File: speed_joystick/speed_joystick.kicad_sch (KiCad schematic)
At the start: 10 parts, among them J1 Conn_01x07, J2 Conn_01x04, SW1 JS5208, U1 Teensy3.2

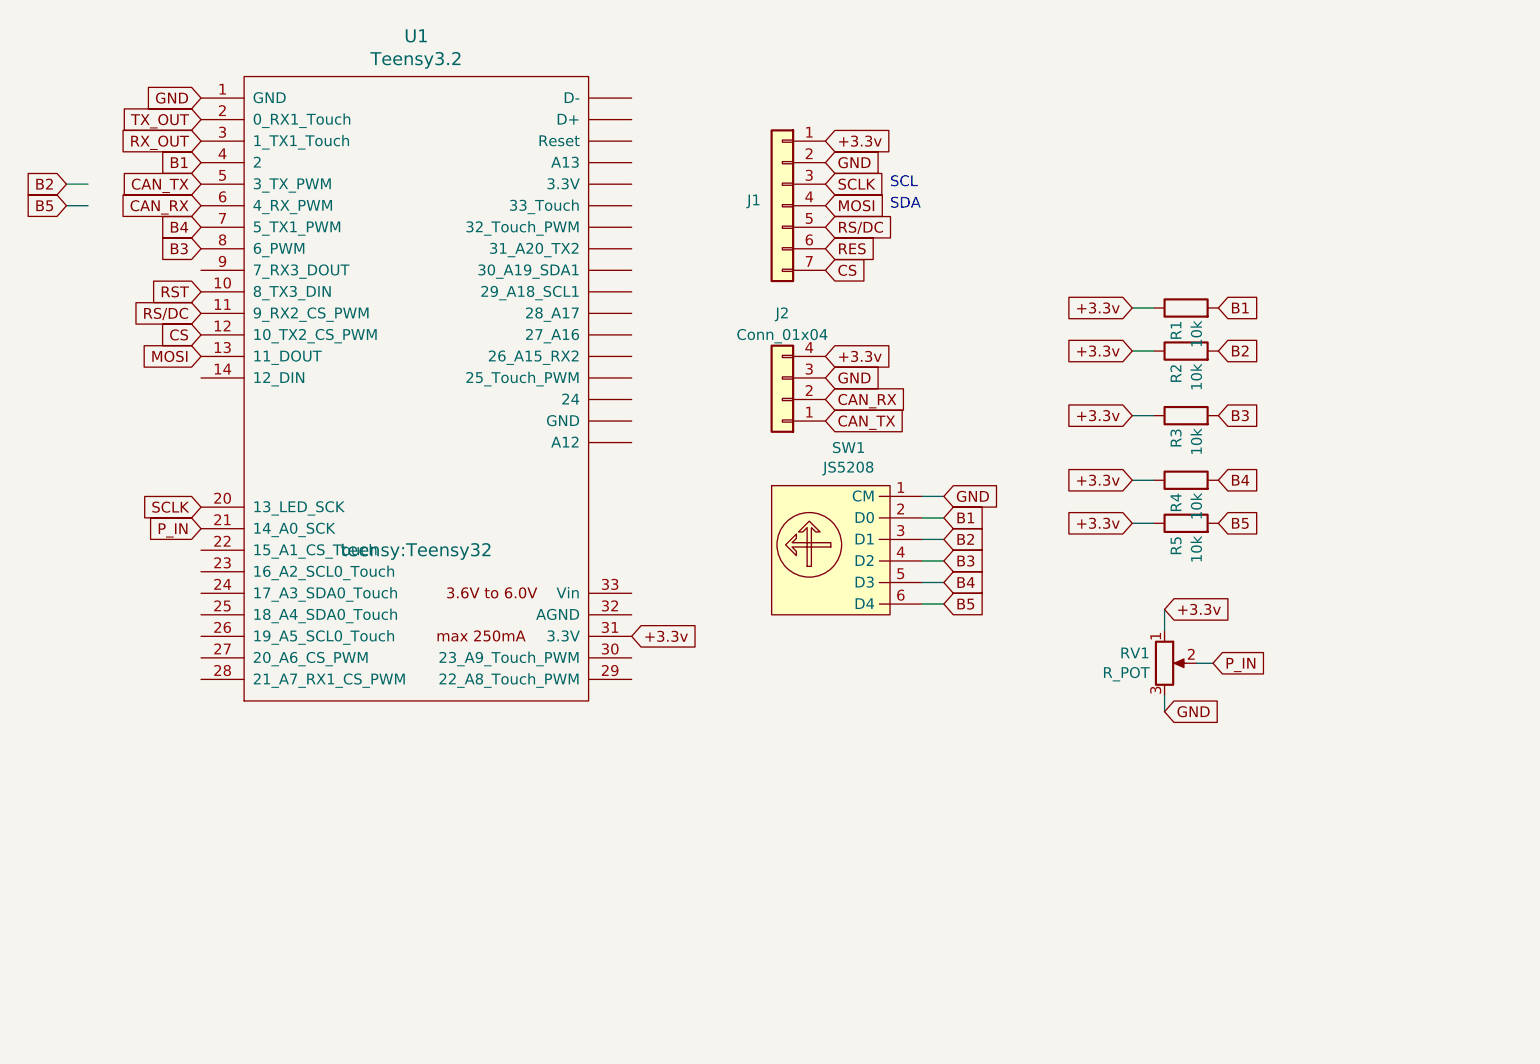
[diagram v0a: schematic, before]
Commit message: pcb work
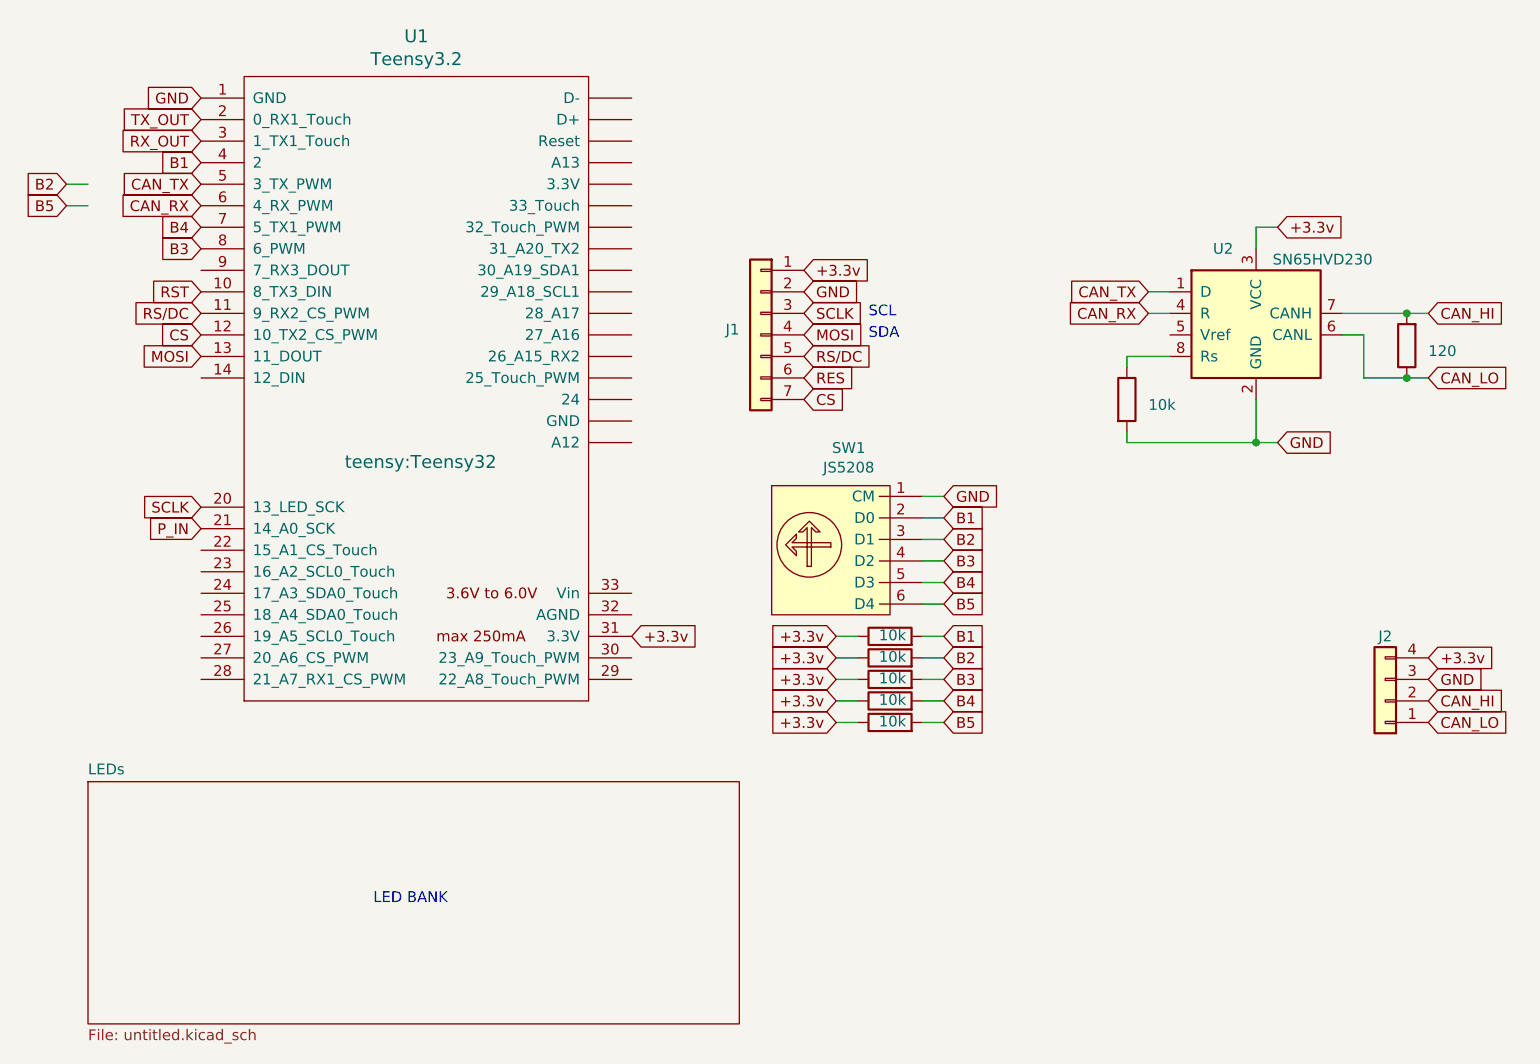
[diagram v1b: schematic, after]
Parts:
- removed RV1: R_POT, Potentiometer_SMD:slide_pot, symbol speed_joystick-rescue:R_POT-Device
- added R6, R7: 10k, Resistor_SMD:R_0805_2012Metric, symbol Device:R
- added U2: SN65HVD230, Package_SO:SOIC-8_3.9x4.9mm_P1.27mm, symbol Interface_CAN_LIN:SN65HVD230
- J2: footprint (none) -> Connector_PinSocket_2.54mm:my_4_tab_edge
- R3: value 10k -> 120; Group# 11 -> (none); P/N 755-ESR10EZPF5102 -> (none)
- SW1: footprint Button_Switch_Keyboard:Joy_switch -> JS5208:SW_JS5208
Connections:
- net +3.3v: now also R6.1, U2.3 (VCC); no longer R3.1
- net B1: now also R6.2; no longer R1.2
- net B2: now also R5.2; no longer R2.2
- net B3: now also R4.2; no longer R3.2
- net B4: now also R2.2; no longer R4.2
- net B5: now also R1.2; no longer R5.2
- net CAN_RX: now also U2.4 (R); no longer J2.2 (Pin_2)
- net CAN_TX: now also U2.1 (D); no longer J2.1 (Pin_1)
- net GND: now also R7.2, U2.2 (GND)
- new net: R7.1, U2.8 (Rs)
- new net CAN_HI: J2.2 (Pin_2), R3.2, U2.7 (CANH)
- new net CAN_LO: J2.1 (Pin_1), R3.1, U2.6 (CANL)
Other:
- added sheet LEDs (untitled.kicad_sch)
- note added: "LED BANK"
- moved on the sheet: J1, J2

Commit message: work on speed_joystick pcb
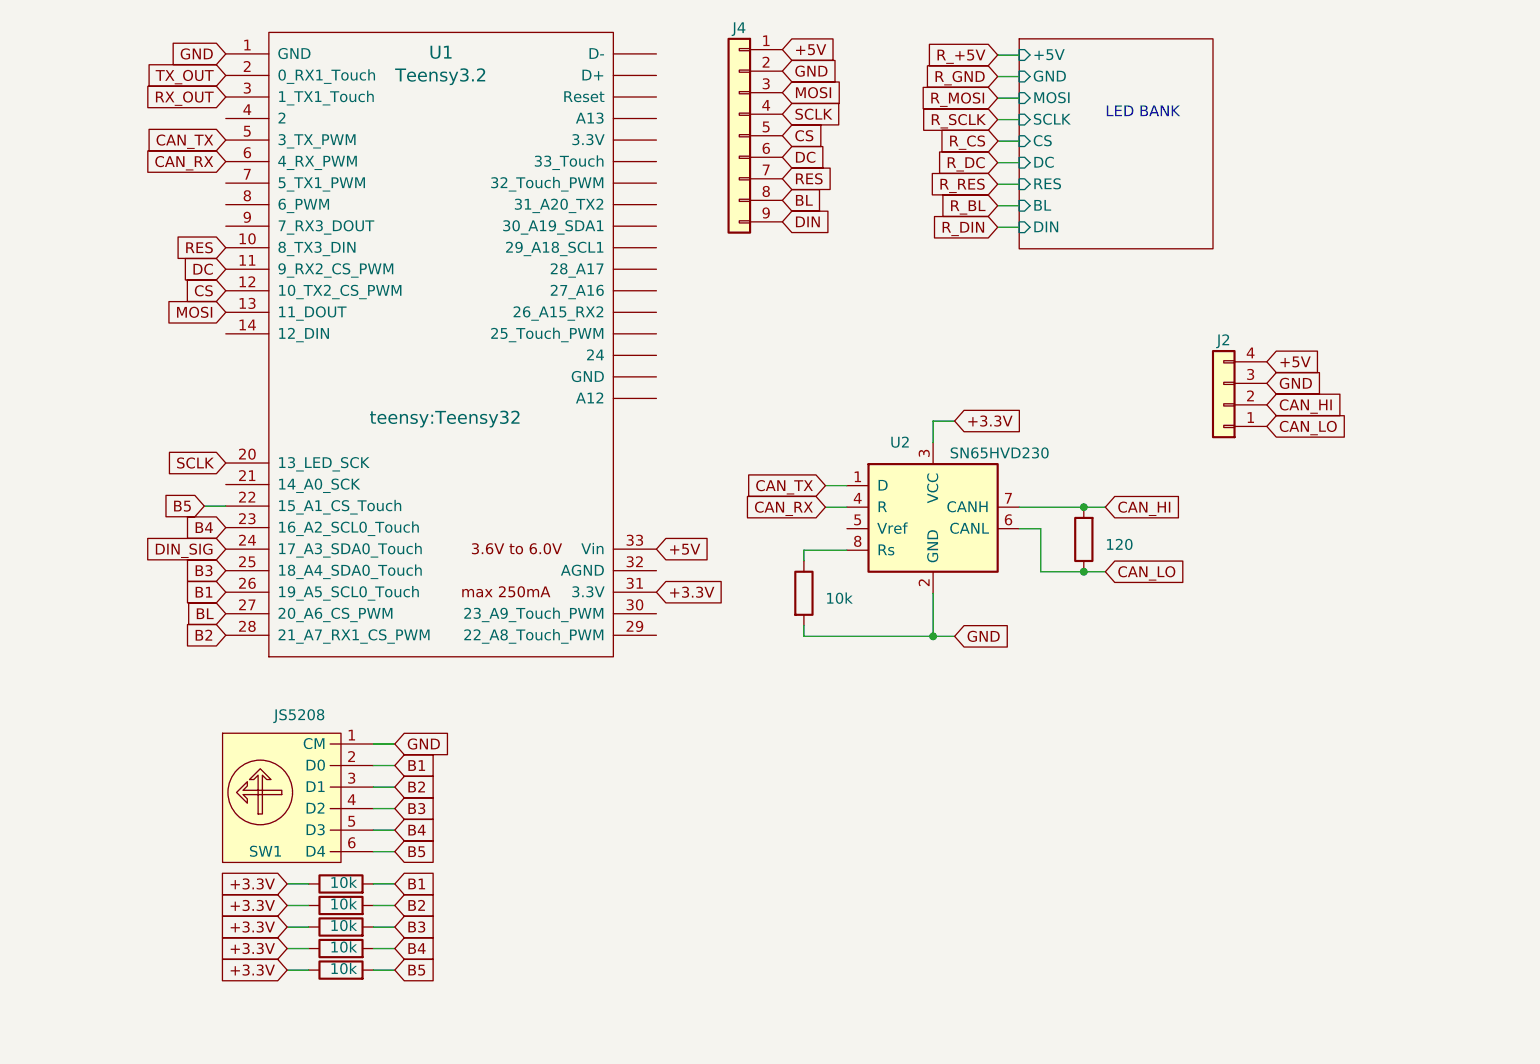
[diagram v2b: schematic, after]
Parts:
- removed J1: Conn_01x07, symbol Connector_Generic:Conn_01x07
- added J4: Conn_01x09, Connector_PinSocket_2.54mm:PinSocket_1x09_P2.54mm_Vertical, symbol Connector_Generic:Conn_01x09
- J2: footprint Connector_PinSocket_2.54mm:my_4_tab_edge -> 4pin:my_4_tab_edge
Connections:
- net RST is gone; now on net RES: U1.10 (8_TX3_DIN)
- net B1: now also U1.26 (19_A5_SCL0_Touch); no longer U1.4 (2)
- net B2: now also U1.28 (21_A7_RX1_CS_PWM)
- net B3: now also U1.25 (18_A4_SDA0_Touch); no longer U1.8 (6_PWM)
- net B4: now also U1.23 (16_A2_SCL0_Touch); no longer U1.7 (5_TX1_PWM)
- net B5: now also U1.22 (15_A1_CS_Touch)
- net CS: now also J4.5 (Pin_5)
- net GND: now also J4.2 (Pin_2)
- net MOSI: now also J4.3 (Pin_3)
- net RES: now also J4.7 (Pin_7)
- net SCLK: now also J4.4 (Pin_4)
- net DIN_SIG: now reaches U1.24 (17_A3_SDA0_Touch)
- net BL: now reaches U1.27 (20_A6_CS_PWM)
- net BL: now also J4.8 (Pin_8)
- net +5V: now reaches U1.33 (Vin)
- net +5V: now also J2.4 (Pin_4), J4.1 (Pin_1)
- net +3.3v renamed +3.3V
- net +3.3V: no longer J2.4 (Pin_4)
- net P_IN: no longer names the net of U1.21 (14_A0_SCK)
- net RS/DC renamed DC
- net DC: now also J4.6 (Pin_6)
- new net DIN: J4.9 (Pin_9)
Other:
- sheet LEDs ports: added +5V, BL, CS, DC, DIN, GND, MOSI, RES, SCLK; removed none
- note removed: "SCL"
- note removed: "SDA"
- moved on the sheet: J2, SW1, U1, U2

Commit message: more round oled work
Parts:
- renumbered R7 to R3, R3 to R7
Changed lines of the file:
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@@
   (symbol (lib_id "Device:R") (at 106.68 86.36 0) (unit 1)
     (in_bom yes) (on_board yes) (dnp no) (fields_autoplaced)
-    (property "Reference" "R7" (at 104.14 86.995 0)
+    (property "Reference" "R3" (at 104.14 86.995 0)
       (effects (font (size 1.27 1.27)) (justify right) hide)
     )
@@
       (project "speed_joystick"
         (path "/4a59a5af-ed4b-4cb8-b8a2-3b43f8ee3aeb"
-          (reference "R7") (unit 1)
+          (reference "R3") (unit 1)
         )
       )
@@
   (symbol (lib_id "Device:R") (at 139.7 80.01 180) (unit 1)
     (in_bom yes) (on_board yes) (dnp no) (fields_autoplaced)
-    (property "Reference" "R3" (at 142.24 79.375 0)
+    (property "Reference" "R7" (at 142.24 79.375 0)
       (effects (font (size 1.27 1.27)) (justify right) hide)
     )
@@
       (project "speed_joystick"
         (path "/4a59a5af-ed4b-4cb8-b8a2-3b43f8ee3aeb"
-          (reference "R3") (unit 1)
+          (reference "R7") (unit 1)
         )
       )
